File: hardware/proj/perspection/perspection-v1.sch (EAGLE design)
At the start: 269 parts, among them J1 MICRO-USB-10118192-0001LF, J10 1X5, J2 1X6-PTSA_1.5/6-3.5-Z, J3 1X2-PTSA_1.5/2-3.5-Z, J4 1X2-JST-PH-SMD, J5 1X2-0428202213, J6 JTAG-ARM_TC-10, J7 JTAG-ARM_TC-10, J8 1X3-0.1IN_THRUHOLE, J9 1X2-PTSA_1.5/2-3.5-Z, Q1 NMOS-CSD18533Q5A, Q10 NMOS-CSD18533Q5A, Q11 IRFML8244TRPBF, Q2 NMOS-CSD18533Q5A, Q3 NMOS-CSD18533Q5A, Q4 NMOS-CSD18533Q5A, Q5 NMOS-CSD18533Q5A, Q6 NMOS-CSD18533Q5A, Q7 NMOS-CSD18533Q5A, Q8 BSS138L, Q9 BSS138L, U1 ATUM, U10 DRV8301DCAR, U11 OPA2374AIDCNR, U12 OPA170AIDBVR, U13 BNO055, U14 TPS81256, U2 FT232RQ, U3 TPS79933DDCR, U4 MCP73831T-2ACI/OT, U5 TMS320F28069MPZT, U6 DRV8801PWPR, U7 DRV8801PWPR, U8 DRV8801PWPR, U9 DRV8801PWPR, Y1 32.768kHz

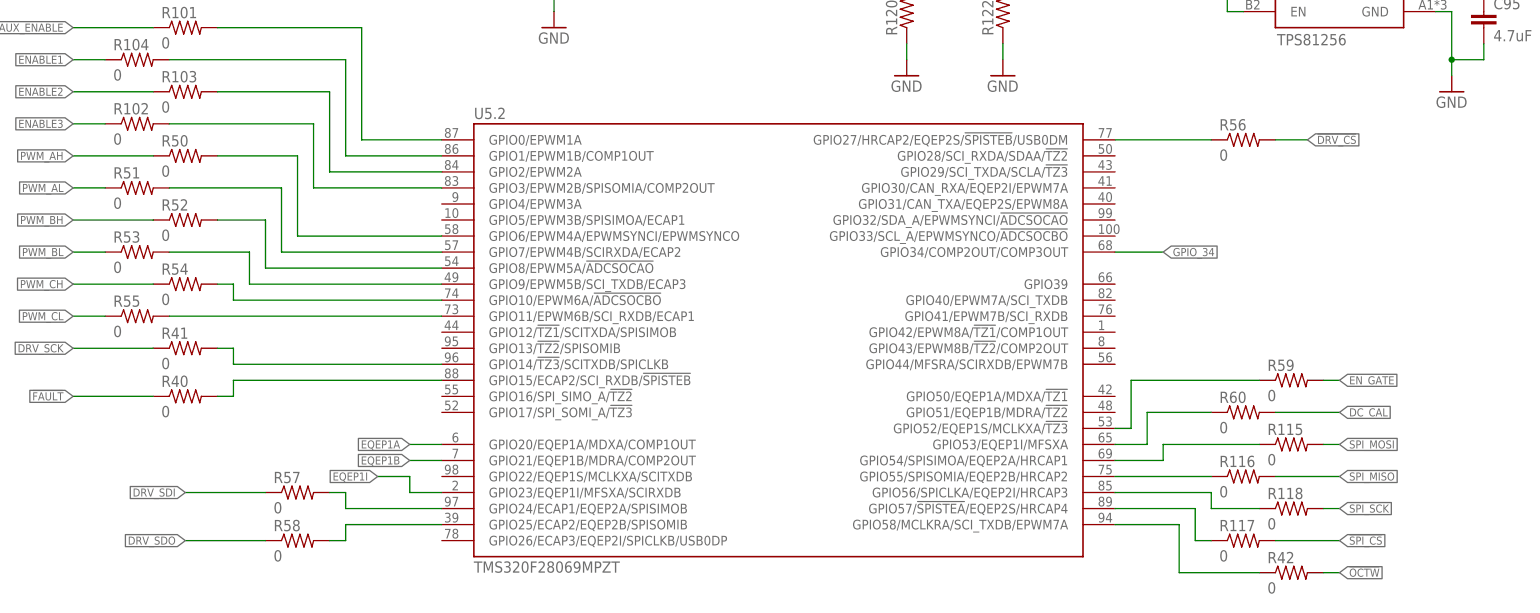
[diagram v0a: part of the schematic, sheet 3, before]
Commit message: pretty much done, need to compile BOM
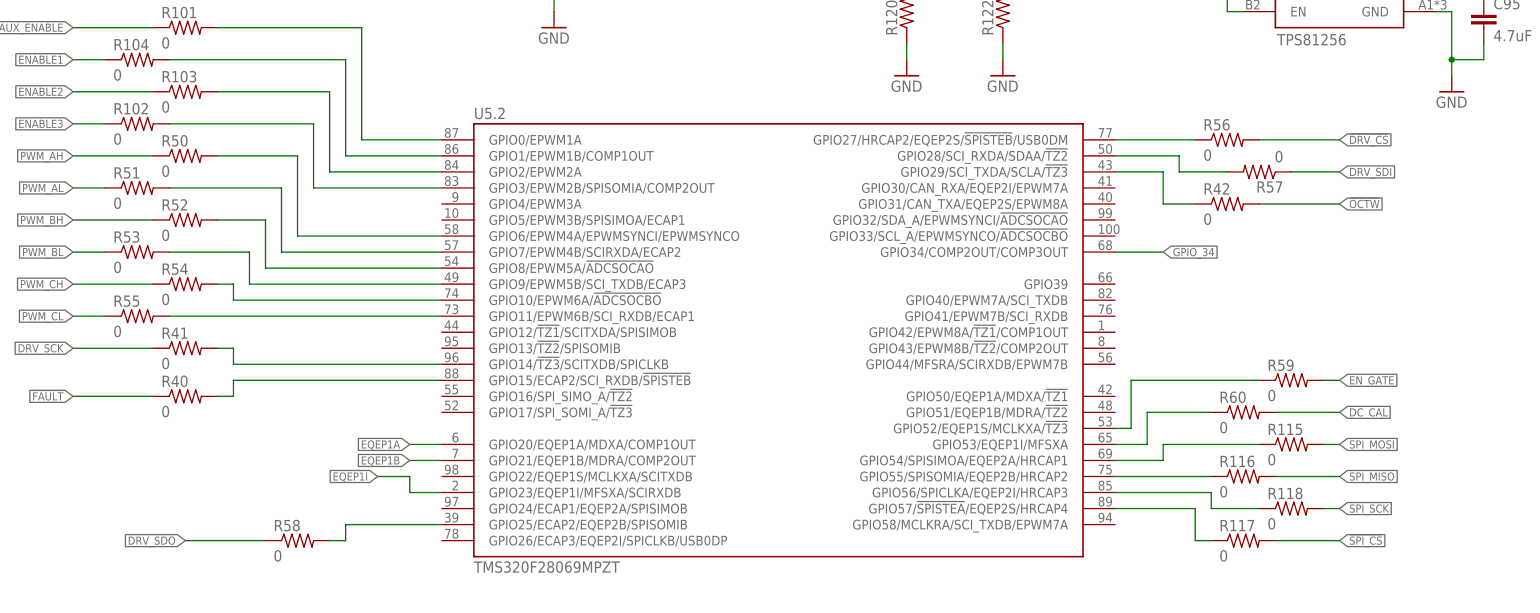
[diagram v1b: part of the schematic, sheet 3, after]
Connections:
- removed net _!OCTW: R42.1, U5.2.GPIO58/MCLKRA/SCI_TXDB/EPWM7A
- removed net _DRV_SDI: R57.2, U5.2.GPIO24/ECAP1/EQEP2A/SPISIMOB
- new net N$21: R57.2, U5.2.GPIO28/SCI_RXDA/SDAA/!TZ2
- new net N$49: R42.1, U5.2.GPIO29/SCI_TXDA/SCLA/!TZ3
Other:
- moved on the sheet: R42, R56, R57
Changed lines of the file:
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@@
 <instance part="R40" gate="G$1" x="78.74" y="45.72"/>
 <instance part="R41" gate="G$1" x="78.74" y="53.34"/>
-<instance part="R42" gate="G$1" x="254" y="17.78"/>
+<instance part="R42" gate="G$1" x="243.84" y="76.2"/>
 <instance part="R43" gate="G$1" x="314.96" y="167.64"/>
 <instance part="R44" gate="G$1" x="314.96" y="157.48"/>
@@
 <instance part="R54" gate="G$1" x="78.74" y="63.5"/>
 <instance part="R55" gate="G$1" x="71.12" y="58.42"/>
-<instance part="R56" gate="G$1" x="246.38" y="86.36"/>
-<instance part="R57" gate="G$1" x="96.52" y="30.48"/>
+<instance part="R56" gate="G$1" x="243.84" y="86.36"/>
+<instance part="R57" gate="G$1" x="248.92" y="81.28" rot="R180"/>
 <instance part="R58" gate="G$1" x="96.52" y="22.86"/>
 <instance part="R59" gate="G$1" x="254" y="48.26"/>
@@
 </segment>
 </net>
-<net name="_!OCTW" class="0">
-<segment>
-<pinref part="U5" gate=".2" pin="GPIO58/MCLKRA/SCI_TXDB/EPWM7A"/>
-<pinref part="R42" gate="G$1" pin="1"/>
-<wire x1="248.92" y1="17.78" x2="236.22" y2="17.78" width="0.1524" layer="91"/>
-<wire x1="236.22" y1="17.78" x2="236.22" y2="25.4" width="0.1524" layer="91"/>
-<wire x1="236.22" y1="25.4" x2="226.06" y2="25.4" width="0.1524" layer="91"/>
-</segment>
-</net>
 <net name="_DC_V_FB" class="0">
 <segment>
@@
 <pinref part="U5" gate=".2" pin="GPIO27/HRCAP2/EQEP2S/!SPISTEB!/USB0DM"/>
 <pinref part="R56" gate="G$1" pin="1"/>
-<wire x1="241.3" y1="86.36" x2="226.06" y2="86.36" width="0.1524" layer="91"/>
-</segment>
-</net>
-<net name="_DRV_SDI" class="0">
-<segment>
-<pinref part="U5" gate=".2" pin="GPIO24/ECAP1/EQEP2A/SPISIMOB"/>
-<pinref part="R57" gate="G$1" pin="2"/>
-<wire x1="101.6" y1="30.48" x2="104.14" y2="30.48" width="0.1524" layer="91"/>
-<wire x1="104.14" y1="30.48" x2="104.14" y2="27.94" width="0.1524" layer="91"/>
-<wire x1="104.14" y1="27.94" x2="119.38" y2="27.94" width="0.1524" layer="91"/>
+<wire x1="238.76" y1="86.36" x2="226.06" y2="86.36" width="0.1524" layer="91"/>
 </segment>
 </net>
@@
 <segment>
 <pinref part="R57" gate="G$1" pin="1"/>
-<wire x1="91.44" y1="30.48" x2="78.74" y2="30.48" width="0.1524" layer="91"/>
-<label x="78.74" y="30.48" size="1.27" layer="95" rot="R180" xref="yes"/>
+<wire x1="254" y1="81.28" x2="261.62" y2="81.28" width="0.1524" layer="91"/>
+<label x="261.62" y="81.28" size="1.27" layer="95" xref="yes"/>
 </segment>
 </net>
@@
 <segment>
 <pinref part="R42" gate="G$1" pin="2"/>
-<wire x1="259.08" y1="17.78" x2="261.62" y2="17.78" width="0.1524" layer="91"/>
-<label x="261.62" y="17.78" size="1.27" layer="95" xref="yes"/>
+<wire x1="248.92" y1="76.2" x2="261.62" y2="76.2" width="0.1524" layer="91"/>
+<label x="261.62" y="76.2" size="1.27" layer="95" xref="yes"/>
 </segment>
 </net>
@@
 <segment>
 <pinref part="R56" gate="G$1" pin="2"/>
-<wire x1="251.46" y1="86.36" x2="256.54" y2="86.36" width="0.1524" layer="91"/>
-<label x="256.54" y="86.36" size="1.27" layer="95" xref="yes"/>
+<wire x1="248.92" y1="86.36" x2="261.62" y2="86.36" width="0.1524" layer="91"/>
+<label x="261.62" y="86.36" size="1.27" layer="95" xref="yes"/>
 </segment>
 </net>
@@
 </segment>
 </net>
+<net name="N$21" class="0">
+<segment>
+<pinref part="U5" gate=".2" pin="GPIO28/SCI_RXDA/SDAA/!TZ2"/>
+<wire x1="226.06" y1="83.82" x2="236.22" y2="83.82" width="0.1524" layer="91"/>
+<wire x1="236.22" y1="83.82" x2="236.22" y2="81.28" width="0.1524" layer="91"/>
+<wire x1="236.22" y1="81.28" x2="243.84" y2="81.28" width="0.1524" layer="91"/>
+<pinref part="R57" gate="G$1" pin="2"/>
+</segment>
+</net>
+<net name="N$49" class="0">
+<segment>
+<pinref part="U5" gate=".2" pin="GPIO29/SCI_TXDA/SCLA/!TZ3"/>
+<wire x1="226.06" y1="81.28" x2="233.68" y2="81.28" width="0.1524" layer="91"/>
+<wire x1="233.68" y1="81.28" x2="233.68" y2="76.2" width="0.1524" layer="91"/>
+<wire x1="233.68" y1="76.2" x2="238.76" y2="76.2" width="0.1524" layer="91"/>
+<pinref part="R42" gate="G$1" pin="1"/>
+</segment>
+</net>
